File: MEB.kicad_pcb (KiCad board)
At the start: 2 copper layers, 49.8 x 49.8 mm, 44 parts, among them J1 171857-0003, J10 1x4 Header, J2 171856-0002, J3 171857-0003, J4 171856-0002, J5 Header, J6 171856-0002, J7 171857-0003, J8 171856-0004, J9 TLW-104-05-T-D, P1 MSP-EXP430G2ET Interface with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, Q1 2.1V, Q2 2N7000, Q3 2N7000, Q4 TP2104N3-G, SW1 FSM2JSMA, SW2 FSM2JSMA, U1 NCP1117LPST33T3G

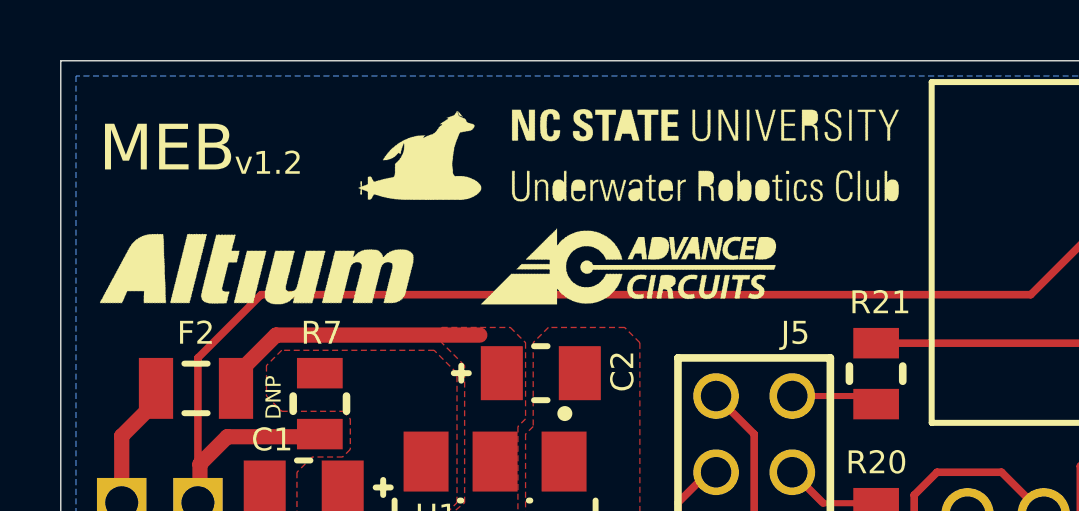
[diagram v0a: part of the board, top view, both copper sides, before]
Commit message: Fix logos
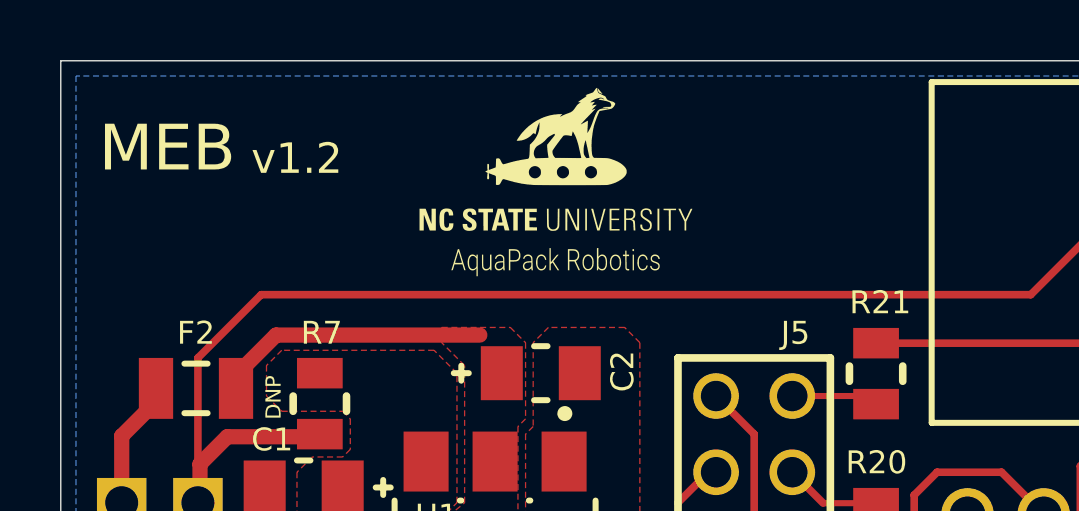
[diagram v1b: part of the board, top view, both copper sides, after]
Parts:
- added G***: LOGO, LOGO, F.Cu at (140.1, 84.2)
